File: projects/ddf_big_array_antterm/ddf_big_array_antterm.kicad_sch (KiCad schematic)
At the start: 75 parts, among them J1 Conn_Coaxial, J101 Conn_Coaxial, J102 Conn_Coaxial, J2 Conn_Coaxial, J201 Conn_Coaxial, J202 Conn_Coaxial, J3 Conn_Coaxial, J301 Conn_Coaxial, J302 Conn_Coaxial, J4 Conn_Coaxial, J401 Conn_Coaxial, J402 Conn_Coaxial, J5 Conn_Coaxial, J6 RJ45_Shielded, J7 RJ45_Shielded, J8 Conn_01x05_Male

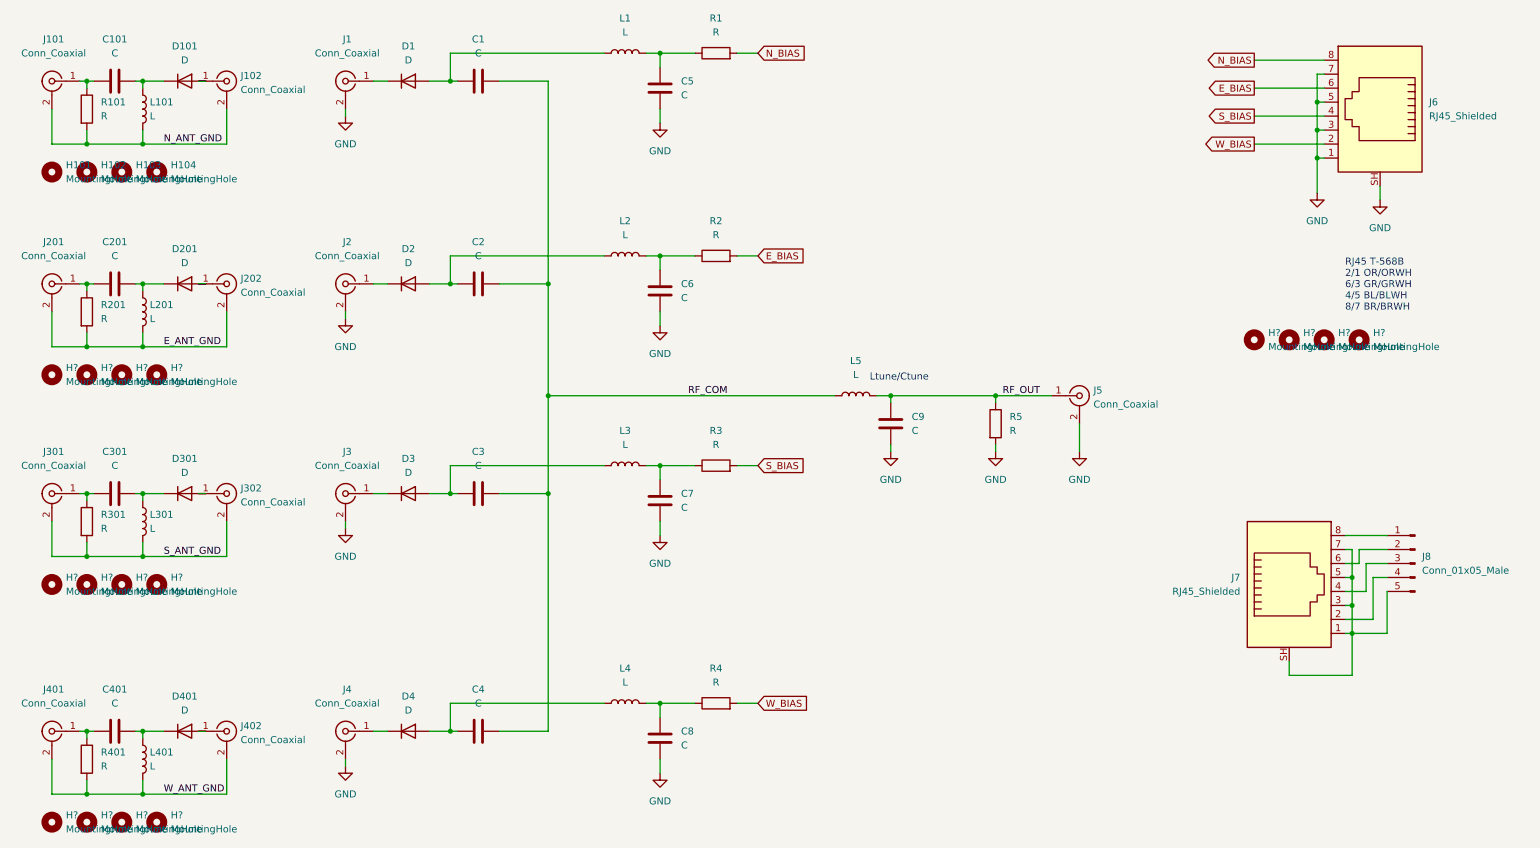
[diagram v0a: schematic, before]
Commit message: Checkpoint.
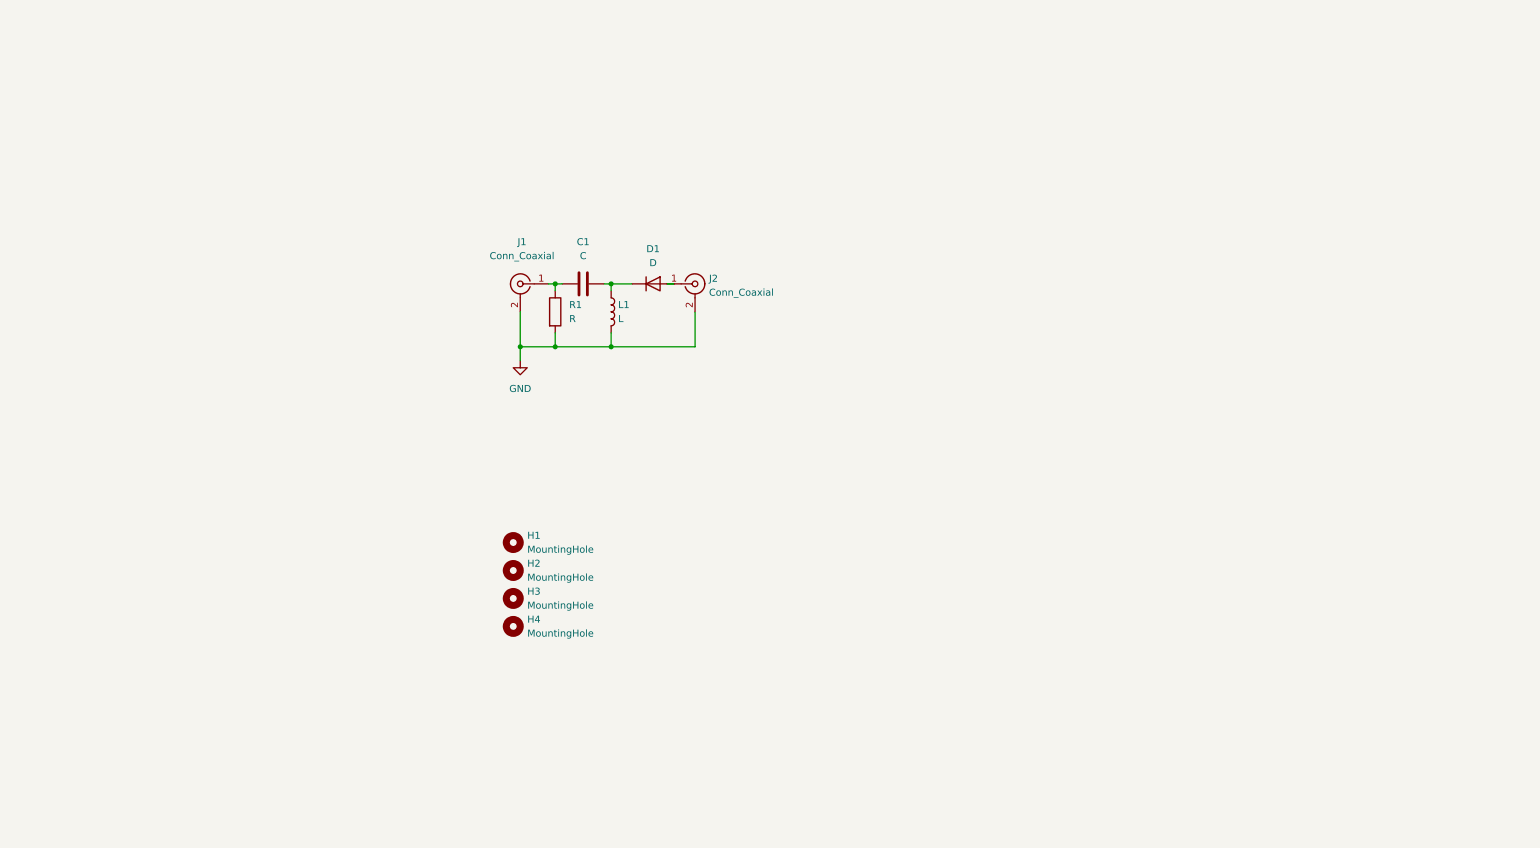
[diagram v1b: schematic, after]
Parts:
- removed C1, C2, C201, C3, C301, C4, C401, C5, C6, C7, C8, C9: C, Capacitor_SMD:C_0402_1005Metric_Pad0.74x0.62mm_HandSolder, symbol Device:C
- removed D1, D2, D201, D3, D301, D4, D401: D, Diode_SMD:D_SOD-523, symbol Device:D
- removed H? (x16): MountingHole, symbol Mechanical:MountingHole
- removed J1, J2, J202, J3, J302, J4, J402: Conn_Coaxial, Connector_Coaxial:SMA_Amphenol_132203-12_Horizontal, symbol Connector:Conn_Coaxial
- removed J201, J301, J401: Conn_Coaxial, Connector_Coaxial:SMA_Amphenol_132134_Vertical, symbol Connector:Conn_Coaxial
- removed J5: Conn_Coaxial, Connector_Coaxial:SMA_Molex_73251-2200_Horizontal, symbol Connector:Conn_Coaxial
- removed J6, J7: RJ45_Shielded, Connector_RJ:RJ45_Wuerth_7499010001A_Horizontal, symbol Connector:RJ45_Shielded
- removed J8: Conn_01x05_Male, Connector_PinHeader_2.54mm:PinHeader_1x05_P2.54mm_Vertical, symbol Connector:Conn_01x05_Male
- removed L1, L2, L201, L3, L301, L4, L401, L5: L, Inductor_SMD:L_0402_1005Metric_Pad0.77x0.64mm_HandSolder, symbol Device:L
- removed R1, R2, R201, R3, R301, R4, R401, R5: R, Resistor_SMD:R_0402_1005Metric_Pad0.72x0.64mm_HandSolder, symbol Device:R
- H1: renamed from H101; footprint (none) -> MountingHole:MountingHole_3.2mm_M3
- H2: renamed from H102; footprint (none) -> MountingHole:MountingHole_3.2mm_M3
- H3: renamed from H103; footprint (none) -> MountingHole:MountingHole_3.2mm_M3
- H4: renamed from H104; footprint (none) -> MountingHole:MountingHole_3.2mm_M3
- renumbered C101 to C1, D101 to D1, J101 to J1, J102 to J2, L101 to L1, R101 to R1
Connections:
- net N_ANT_GND is gone; now on net GND: J1.2 (Ext), J2.2 (Ext), L1.2, R1.2
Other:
- note removed: "Ltune/Ctune"
- note removed: "RJ45 T-568B 2/1 OR/ORWH 6/3 GR/GRWH 4/5 BL/BLWH 8/7 BR/BRWH"
- moved on the sheet: C1, D1, H1, H2, H3, H4, J1, J2, L1, R1
